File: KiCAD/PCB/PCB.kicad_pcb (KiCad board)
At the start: 2 copper layers, 68 x 68 mm, 62 parts, among them J1 Conn_01x04, J2 Conn_01x02, P1 USB_C_Plug, Q1 Q_NPN_EBC, Q2 Q_NPN_EBC, SW1 SW_Push, SW2 SW_Push, SW3 RotaryEncoder_Switch, SW4 SW_Push, SW5 SW_Push, U1 MIC5219-3.3YM5, U2 CH340G, U3 MCP73832-5-OT, U4 ESP32-WROOM-32D, U5 MPU-6050, Y1 12Mhz

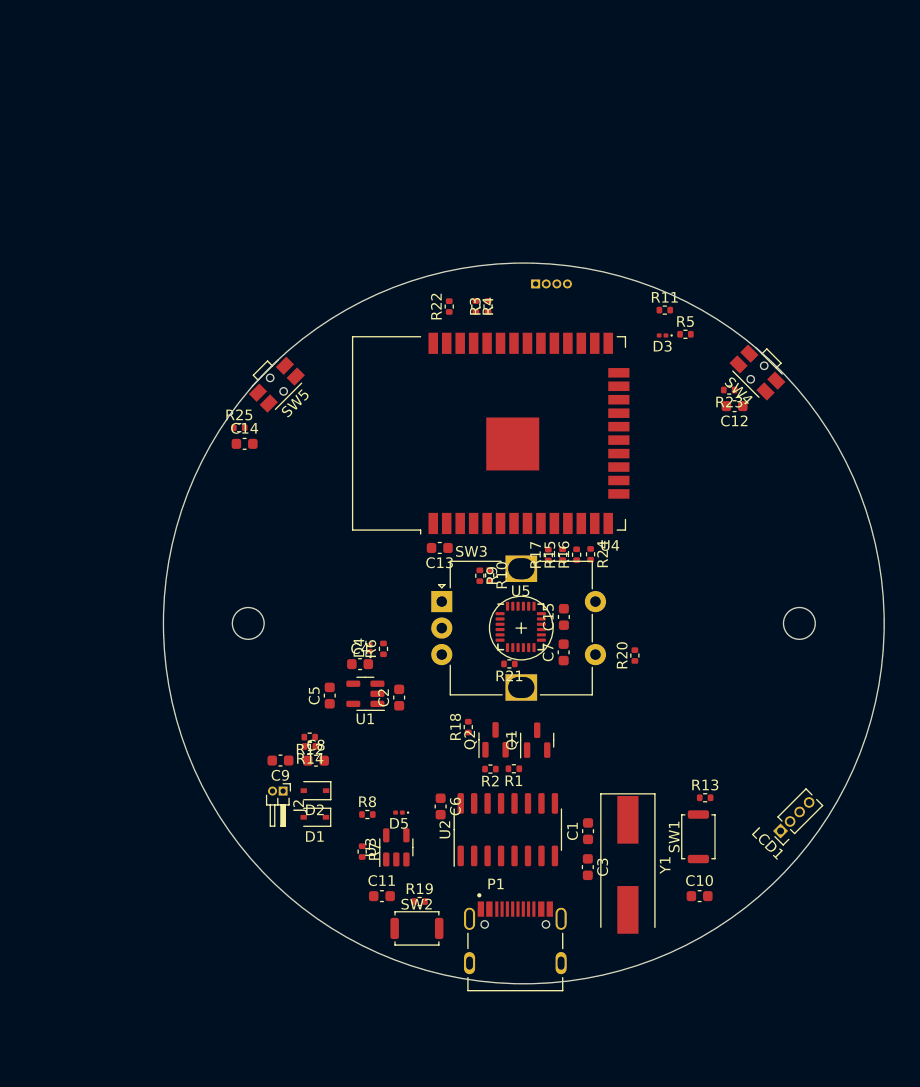
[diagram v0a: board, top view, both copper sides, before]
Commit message: 完成佈線
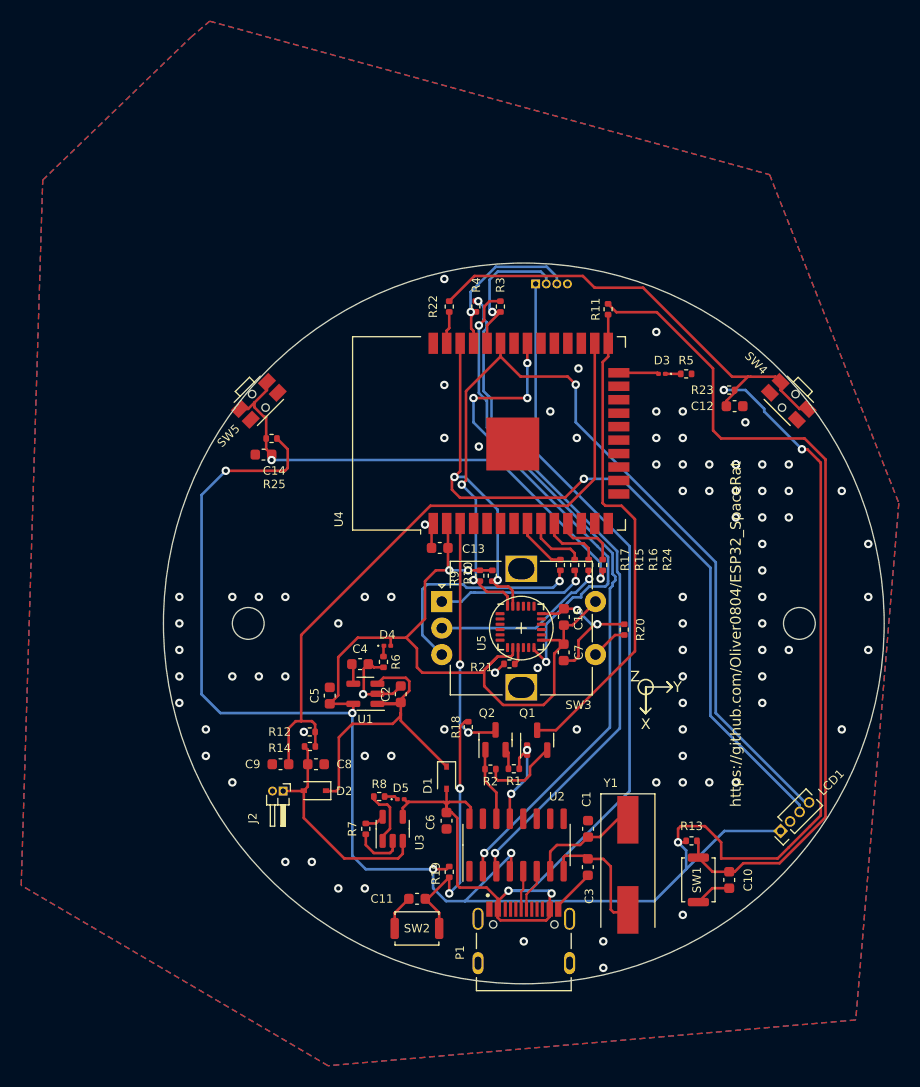
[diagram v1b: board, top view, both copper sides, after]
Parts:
- added V0.1: LOGO, LOGO, B.Cu at (101.0, 82.5)
- moved D1 13.0 mm to (92.7, 114.6), turned to -90 degrees
- moved R11 5.35 mm to (108.0, 70.4), turned to 90 degrees
- moved R13 4.26 mm to (115.8, 120.5)
- moved SW1 4.06 mm to (116.5, 124.2)
- moved SW4 3.98 mm to (125.0, 79.0)
- moved R19 3.95 mm to (93.0, 123.4), turned to -90 degrees
- moved R5 3.73 mm to (115.3, 76.5)
- moved D3 3.62 mm to (113.0, 76.5)
- moved C11 3.32 mm to (89.9, 126.0)
- moved R25 3.21 mm to (76.2, 82.5), turned to 180 degrees
- moved C10 3.18 mm to (119.4, 124.2), turned to 90 degrees
- moved R20 2.64 mm to (109.5, 100.6)
- moved SW5 2.29 mm to (75.0, 79.0)
- moved R7 2.17 mm to (85.1, 119.4)
- moved C14 2.05 mm to (75.4, 84.1)
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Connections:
- LCD1 pad 1: /3V3 -> +3V3
- SW3 pad S1: /3V3 -> +3V3
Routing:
- net +3V3: track 0.00 -> 254.5 mm, vias 0 -> 9
- net +5V: track 0.00 -> 106.9 mm, vias 0 -> 2
- net /LCD_SDA: track 0.00 -> 86.4 mm, vias 0 -> 3
- net /LCD_SCL: track 0.00 -> 85.9 mm, vias 0 -> 3
- net Net-(C10-Pad2): track 0.00 -> 80.1 mm
- net Net-(R3-Pad1): track 0.00 -> 65.7 mm, vias 0 -> 2
- net Net-(R4-Pad1): track 0.00 -> 64.7 mm, vias 0 -> 2
- net /ADC0: track 0.00 -> 63.1 mm
- net Net-(C14-Pad2): track 0.00 -> 47.7 mm, vias 0 -> 2
- net /ESP32_IO0: track 0.00 -> 46.4 mm
- net /MPU_INT: track 0.00 -> 46.0 mm, vias 0 -> 4
- net Net-(C12-Pad2): track 0.00 -> 44.1 mm
- net GND: track 0.00 -> 42.2 mm, vias 0 -> 88
- net Net-(C2-Pad1): track 0.00 -> 30.9 mm
- net Net-(C11-Pad2): track 0.00 -> 25.1 mm, vias 0 -> 2
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- added copper zone on B.Cu, net GND
- added copper zone on F.Cu, net GND
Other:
- board text added: "X"
- board text added: "Y"
- board text added: "Z"
- board text added: "https://github.com/Oliver0804/ESP32_SpaceRat"
